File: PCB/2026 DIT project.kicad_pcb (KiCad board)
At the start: 2 copper layers, 1 part

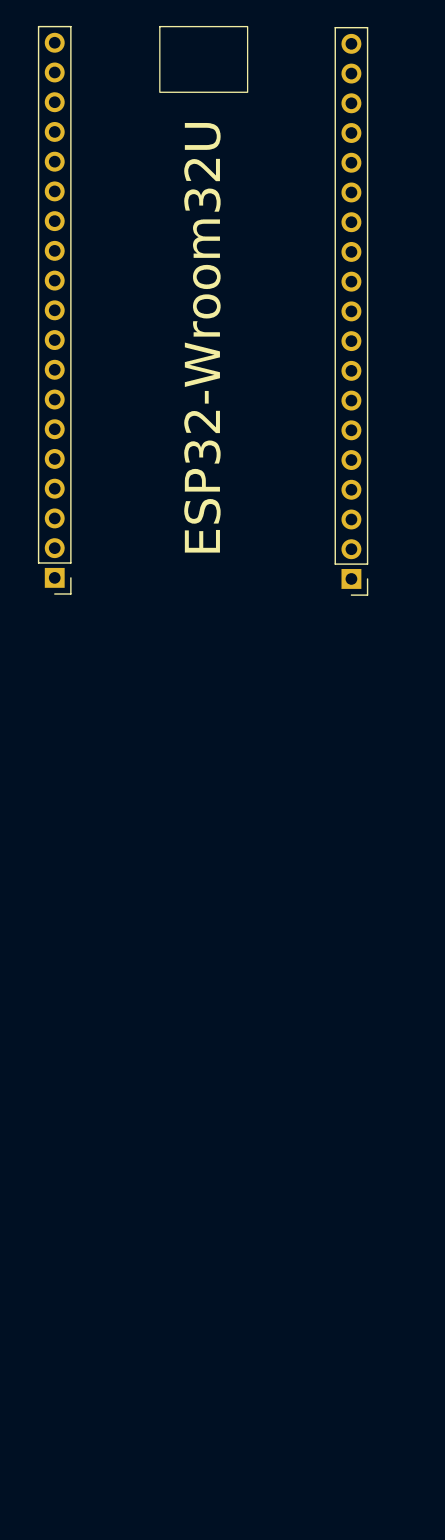
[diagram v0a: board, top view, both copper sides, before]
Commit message: PCB design process
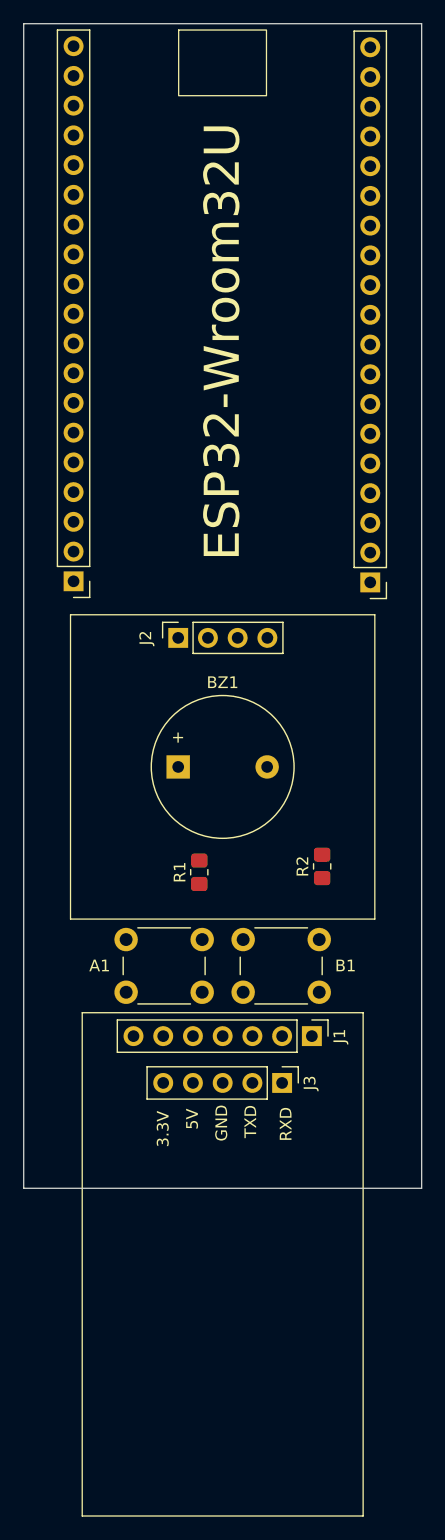
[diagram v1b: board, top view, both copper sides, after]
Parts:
- added A1: SW_Push_Open_Dual, Button_Switch_THT:SW_PUSH_6mm, F.Cu at (31.8, 110.2)
- added B1: SW_Push_Open_Dual, Button_Switch_THT:SW_PUSH_6mm, F.Cu at (41.8, 110.2)
- added BZ1: Buzzer, Buzzer_Beeper:Buzzer_12x9.5RM7.6, F.Cu at (36.2, 95.5)
- added J1: Conn_01x07_Socket, Connector_PinHeader_2.54mm:PinHeader_1x07_P2.54mm_Vertical, F.Cu at (47.6, 118.5)
- added J2: Conn_01x04_Socket, Connector_PinSocket_2.54mm:PinSocket_1x04_P2.54mm_Vertical, F.Cu at (36.2, 84.5)
- added J3: Conn_01x05_Pin, Connector_PinHeader_2.54mm:PinHeader_1x05_P2.54mm_Vertical, F.Cu at (45.1, 122.5)
- added R1: 10k, Resistor_SMD:R_0805_2012Metric_Pad1.20x1.40mm_HandSolder, F.Cu at (38.0, 104.5)
- added R2: 10k, Resistor_SMD:R_0805_2012Metric_Pad1.20x1.40mm_HandSolder, F.Cu at (48.5, 104.0)
- U1: renamed from A1; value ~ -> ESP32-WROOM32U
- moved U1 1.64 mm to (25.5, 32.2)
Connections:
- U1 pad 0: unconnected-(A1-Pad0) -> /Buzzer
- U1 pad 16: unconnected-(A1-Pad16) -> /TXD
- U1 pad 17: unconnected-(A1-Pad17) -> /RXD
- U1 pad 2: unconnected-(A1-Pad2) -> /BTN_A
- U1 pad 21: unconnected-(A1-Pad21) -> /SDA
- U1 pad 22: unconnected-(A1-Pad22) -> /SCL
- U1 pad 3V3: unconnected-(A1-Pad3V3) -> +3V3
- U1 pad 4: unconnected-(A1-Pad4) -> /BTN_B
- U1 pad 5V: Net-(A1-Pad5V) -> +5V
- U1 pad CLK: Net-(A1-Pad5V) -> unconnected-(U1-PadCLK)
- U1 pad GND: unconnected-(A1-PadGND) -> GND
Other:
- board outline added: 34 x 99.5 mm
- board text added: "3.3V"
- board text added: "5V"
- board text added: "GND"
- board text added: "RXD"
- board text added: "TXD"
